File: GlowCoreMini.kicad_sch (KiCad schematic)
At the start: 36 parts, among them J1 Conn_02x03_Counter_Clockwise, J2 DC-042C-Z-2.5-A, P1 WJ15EDGRC-3.81-3P, Q1 AP40P05, Q2 MMBT2222A, Q3 MMBT2222A, Q4 AP40P05, SW1 TS-1185EC-C-D-B, SW2 TS-1185EC-C-D-B, U1 SN74AHCT32QPWRQ1, U2 ESP32-WROOM-32E (4MB), U3 BL1117-33CX, U4 CP2102-GMR

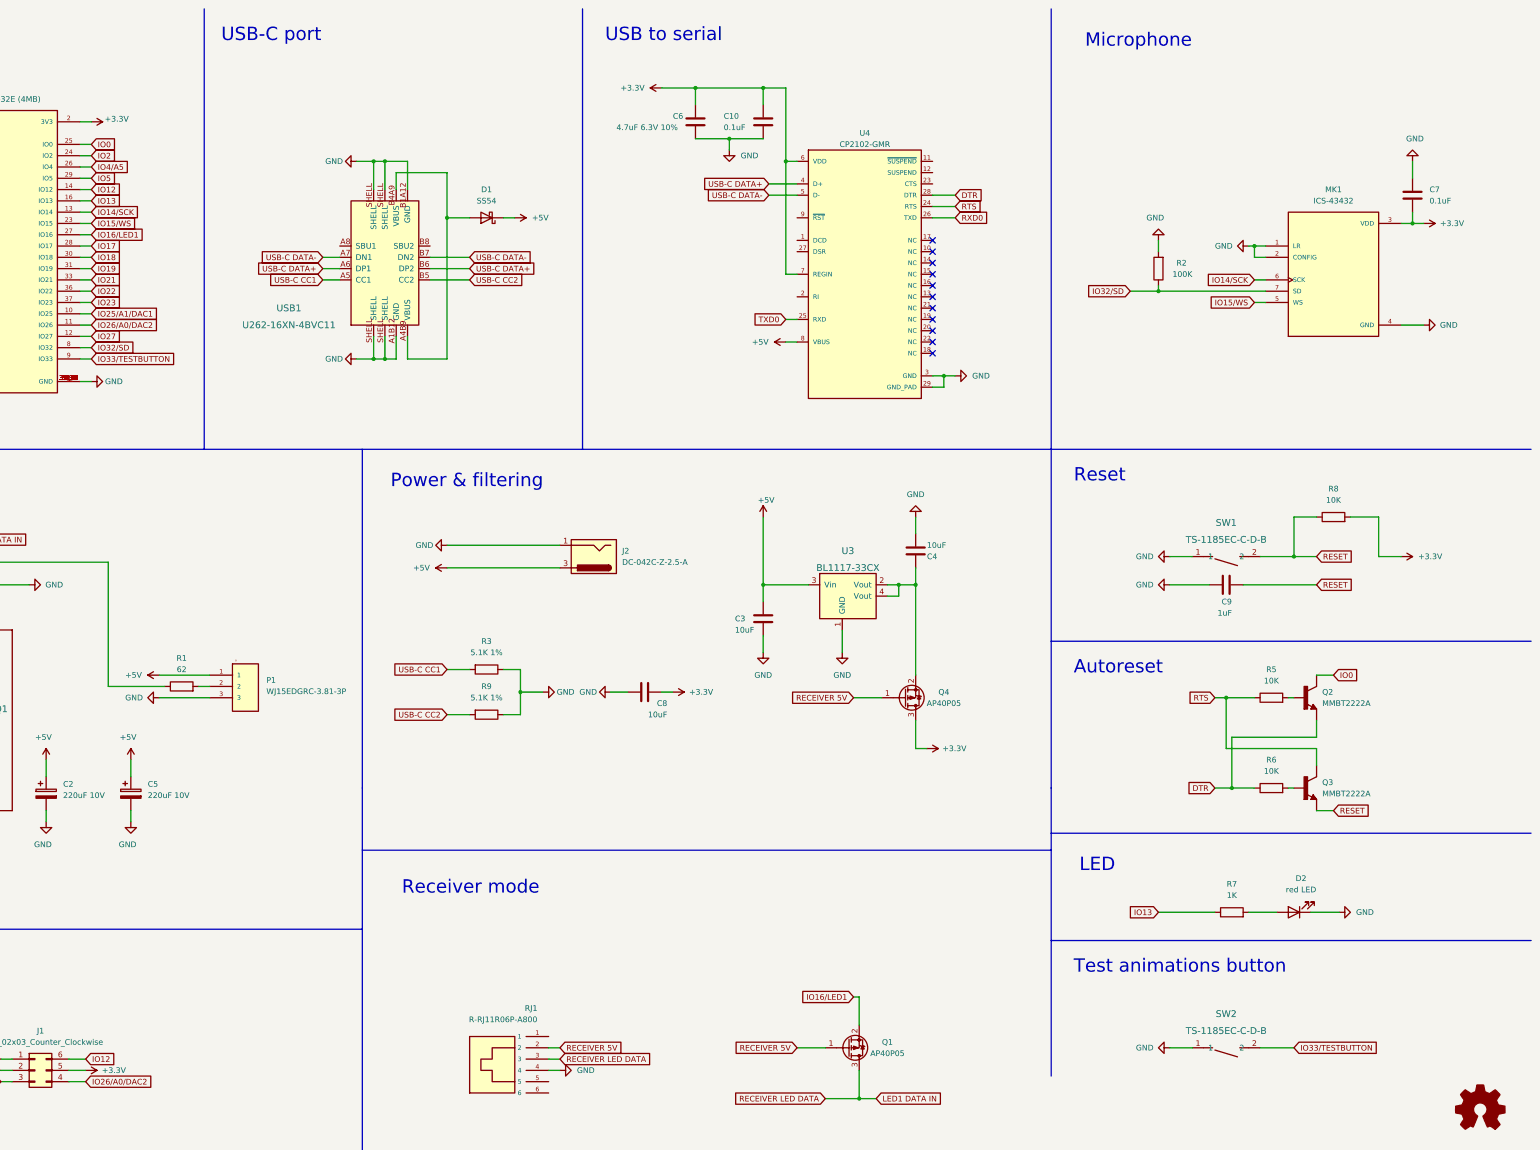
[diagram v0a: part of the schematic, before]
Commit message: add warning info
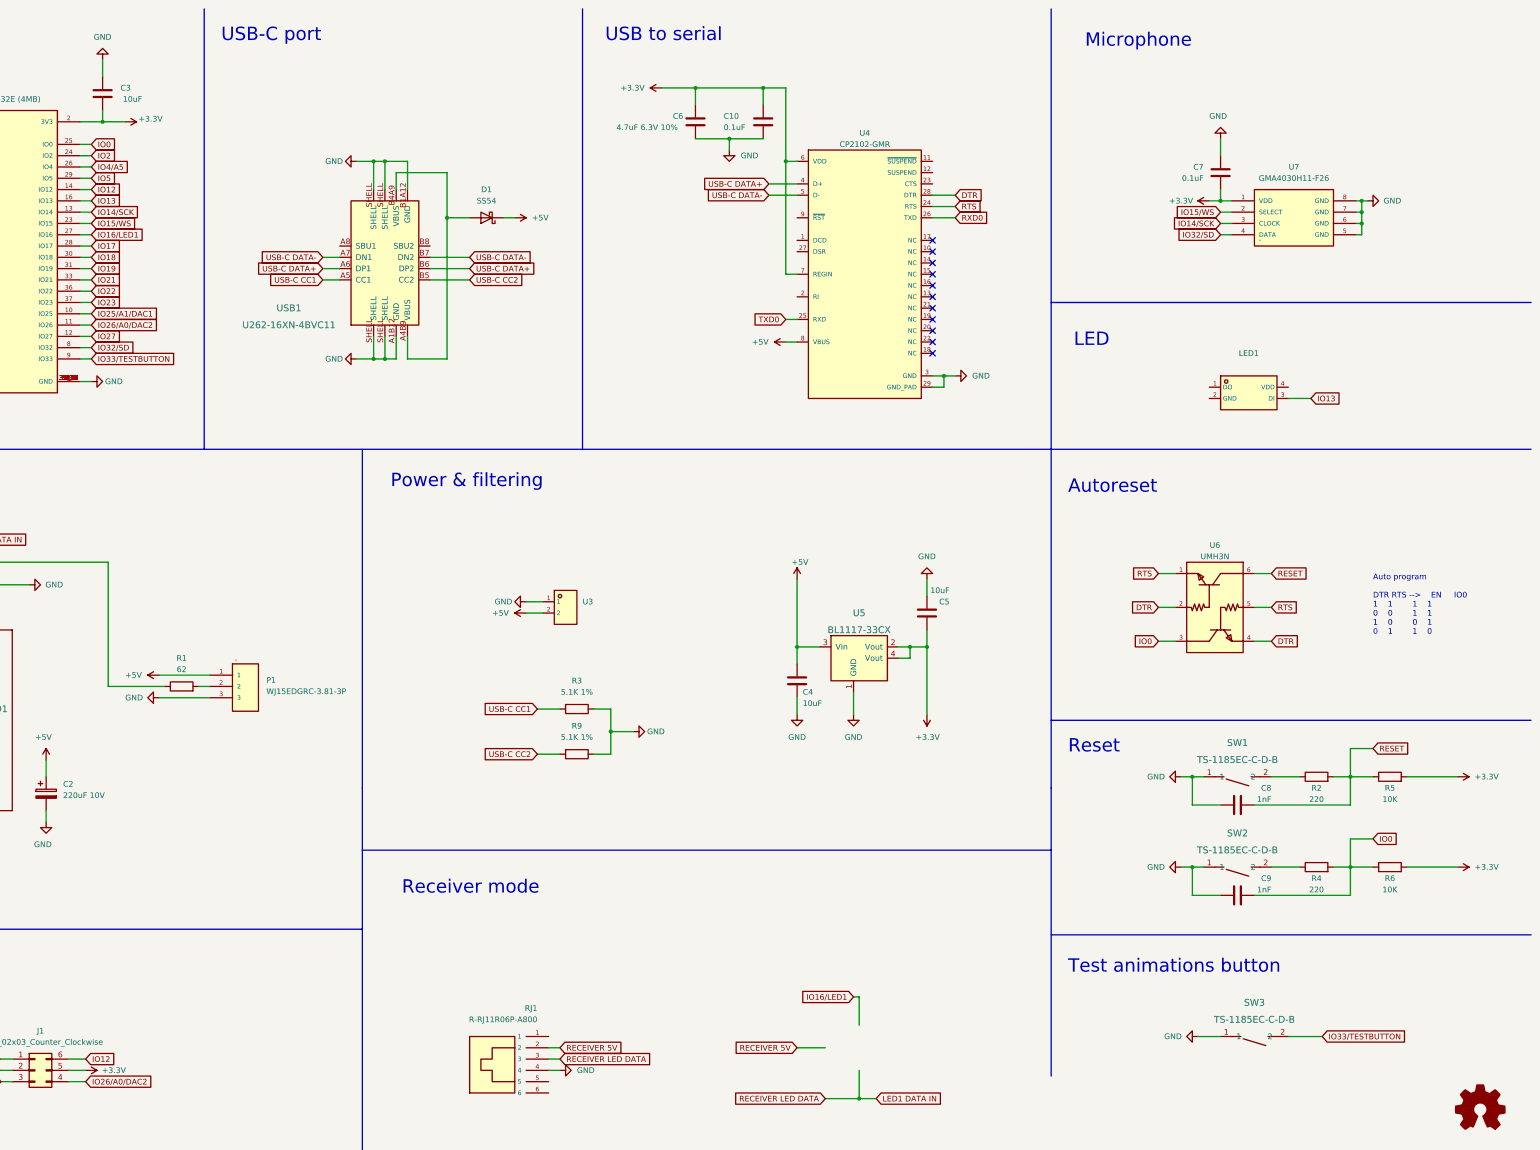
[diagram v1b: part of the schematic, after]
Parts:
- removed C5: 220uF 10V, Capacitor_SMD:CP_Elec_6.3x5.4, symbol Device:220uF 10V 6.3x5.4mm
- removed C9: 1uF, Capacitor_SMD:C_0603_1608Metric_Pad1.08x0.95mm_HandSolder, symbol Device:1uF 0603
- removed D2: red LED, LED_SMD:LED_0603_1608Metric_Pad1.05x0.95mm_HandSolder, symbol Device:red LED 0603
- removed J2: DC-042C-Z-2.5-A, DC-042C-Z-2:DC-IN-TH_DC-042C-Z-2.5-A, symbol Connector:DC-042C-Z-2.5-A
- removed MK1: ICS-43432, ICS-43432:MIC_ICS-43432, symbol ICS-43432:ICS-43432
- removed Q1, Q4: AP40P05, Package_TO_SOT_SMD:SOT-23, symbol Transistor_FET:SK338P
- removed Q2, Q3: MMBT2222A, Package_TO_SOT_SMD:SOT-23, symbol MMBT2222A:MMBT2222A
- removed R2: 100K, Resistor_SMD:R_0603_1608Metric_Pad0.98x0.95mm_HandSolder, symbol Device:100K 0603
- removed R7: 1K, Resistor_SMD:R_0603_1608Metric_Pad0.98x0.95mm_HandSolder, symbol Device:1K_0603
- removed R8: 10K, Resistor_SMD:R_0603_1608Metric_Pad0.98x0.95mm_HandSolder, symbol Device:10K 0603
- removed U3: BL1117-33CX, Package_TO_SOT_SMD:SOT-223, symbol BL1117-33CX:BL1117-33CX
- added C5: 10uF, Capacitor_SMD:C_0603_1608Metric_Pad1.08x0.95mm_HandSolder, symbol Device:10uF 0603
- added C9: 1nF, Capacitor_SMD:C_0603_1608Metric_Pad1.08x0.95mm_HandSolder, symbol Device:10uF 0603
- added LED1: (no value), symbol LCSC:WS2812B-2020
- added R2, R4: 220, Resistor_SMD:R_0603_1608Metric_Pad0.98x0.95mm_HandSolder, symbol Device:10K 0603
- added SW3: TS-1185EC-C-D-B, TS-1185EC-C-D-B:TS-1185EC-C-D-B, symbol TS-1185EC-C-D-B:TS-1185EC-C-D-B
- added U3: (no value), symbol LCSC:KF350-3_5-2P
- added U5: BL1117-33CX, Package_TO_SOT_SMD:SOT-223, symbol BL1117-33CX:BL1117-33CX
- added U6: UMH3N, footprint:SC-70-6_L2.2-W1.3-P0.65-LS2.1-BR, symbol LCSC:UMH3N
- added U7: GMA4030H11-F26, GMA4030H11-F26:GMA4030H11-F26, symbol GMA4030H11-F26:GMA4030H11-F26
- C8: value 10uF -> 1nF
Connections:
- net +3V3: now also C3.2, R5.2, R6.2, C5.2, U5.2 (Vout), U5.4 (Vout), U7.1 (VDD); no longer C8.1
- net +5V: now also C4.2, U3.2, U5.3 (Vin); no longer C3.2
- net DTR: now also U6.2 (B), U6.4 (E); no longer R6.1
- net GND: now also C5.1, C9.2, SW3.1, U3.1, U5.1 (GND), U7.5 (GND), U7.6 (GND), U7.7 (GND), U7.8 (GND)
- net IO0: now also R6.1, C9.1, R4.2, U6.3 (C)
- net IO13: now also LED1.3 (DI)
- net IO14/SCK: now also U7.3 (CLOCK)
- net IO15/WS: now also U7.2 (SELECT)
- net IO32/SD: now also U7.4 (DATA)
- net IO33/TESTBUTTON: now also SW3.2; no longer SW2.2
- net RESET: now also C8.1, R5.1, R2.2, U6.6 (C); no longer SW1.2
- net RTS: now also U6.1 (E), U6.5 (B); no longer R5.1
- new net: R4.1, SW2.2
- new net: R2.1, SW1.2
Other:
- note added: "Auto program DTR RTS --> EN IO0 1 1 1 1 0 0 1 1 1 0 0 1 0 1 1 0"
- moved on the sheet: R3, R9
